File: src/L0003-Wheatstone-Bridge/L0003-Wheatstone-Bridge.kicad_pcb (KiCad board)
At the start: 2 copper layers, 63.5 x 22.9 mm, 18 parts, among them P1 12V, P2 2043-1X04G00DAU, U1 MCP1703T-4002E_DB

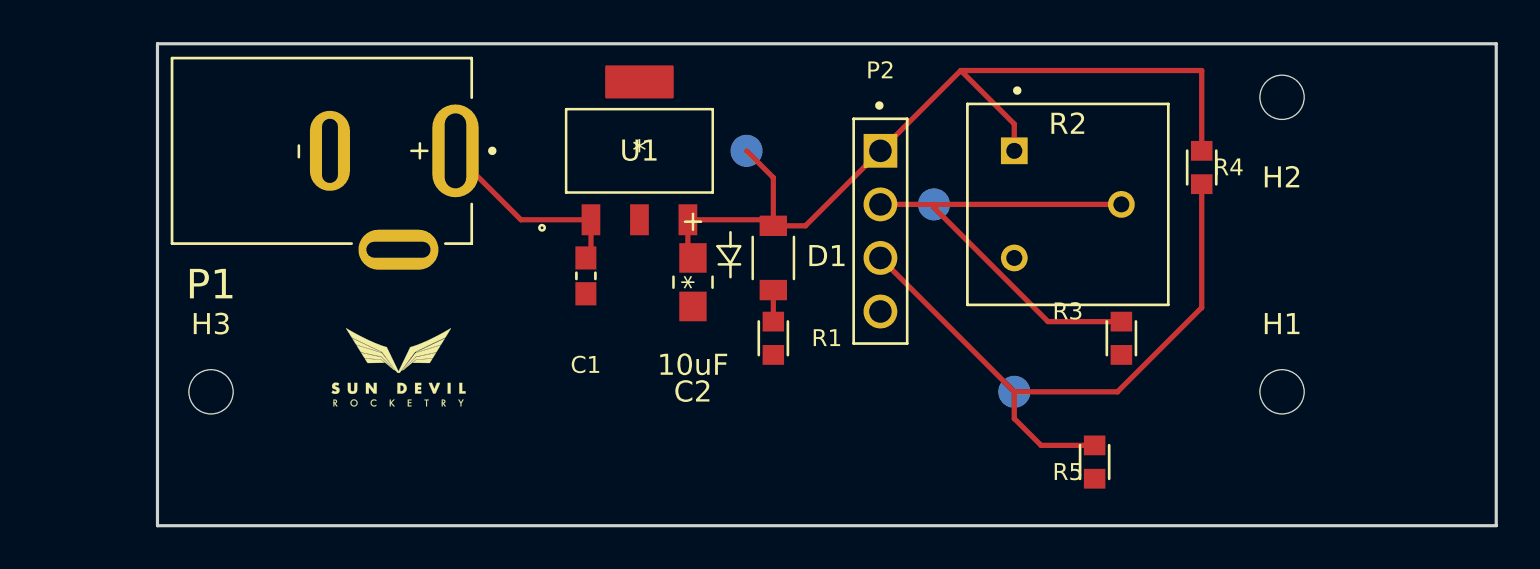
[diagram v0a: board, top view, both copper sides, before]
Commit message: Finished PCB
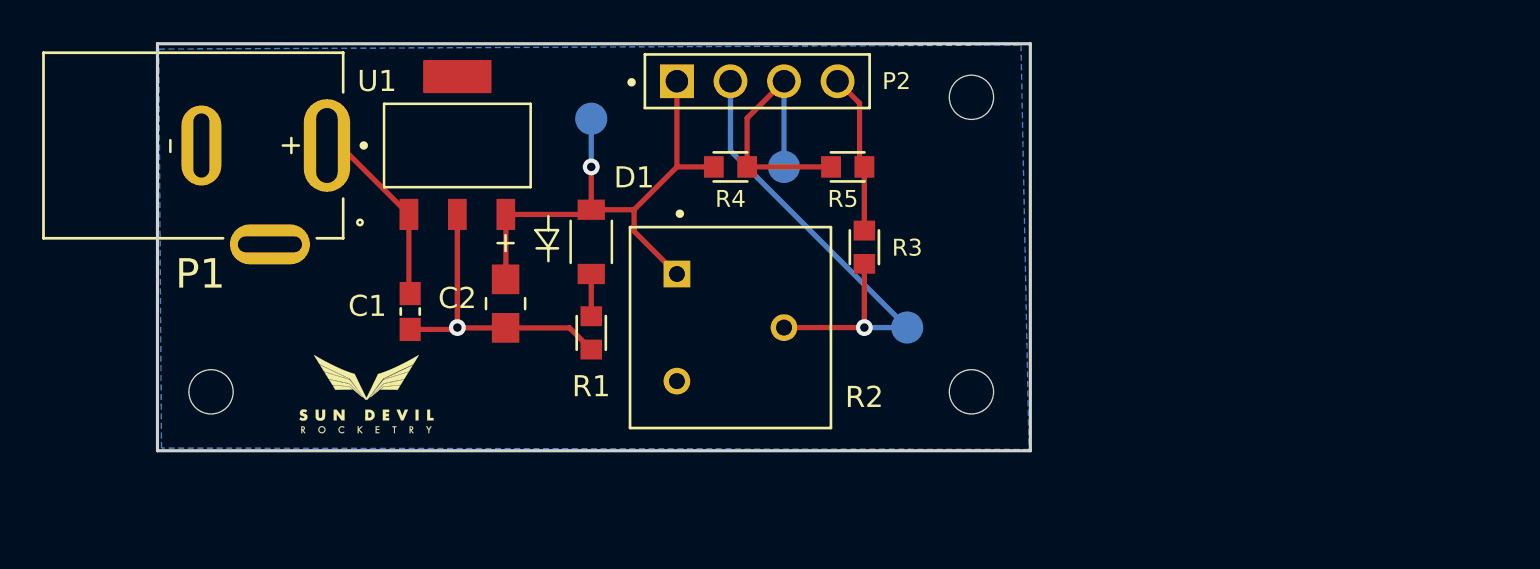
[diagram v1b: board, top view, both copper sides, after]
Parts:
- moved R4 22.4 mm to (122.4, 82.0), turned to 0 degrees
- moved R5 18.3 mm to (128.0, 82.0), turned to 0 degrees
- moved R2 17.0 mm to (122.4, 89.7)
- moved TP3 15.3 mm to (125.0, 82.0)
- moved H1 14.7 mm to (133.9, 92.7)
- moved H2 14.7 mm to (133.9, 78.7)
- moved R3 12.9 mm to (128.8, 85.9), turned to 90 degrees
- moved P2 9.20 mm to (123.7, 78.0), turned to 0 degrees
- moved C2 8.95 mm to (111.8, 88.5)
- moved D1 8.67 mm to (115.8, 85.6)
- moved R1 8.64 mm to (115.8, 89.9)
- moved U1 8.64 mm to (109.5, 81.0)
- moved C1 8.50 mm to (107.2, 88.9)
- moved TP1 7.52 mm to (115.8, 79.8)
- moved P1 6.10 mm to (100.6, 81.0)
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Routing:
- net Earth: track 0.00 -> 23.4 mm, vias 0 -> 1
- net Vout-: track 31.0 -> 12.8 mm
- net +5V: track 42.2 -> 26.2 mm, vias 0 -> 1
- net Vout+: track 22.7 -> 24.0 mm, vias 0 -> 1
- net Net-(D1-Pad1): track 1.50 -> 2.00 mm
- added copper zone on B.Cu, net Earth
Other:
- board size 63.5 x 22.9 mm -> 41.4 x 19.3 mm
